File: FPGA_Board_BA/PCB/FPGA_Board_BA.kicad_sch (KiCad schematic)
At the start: 0 parts

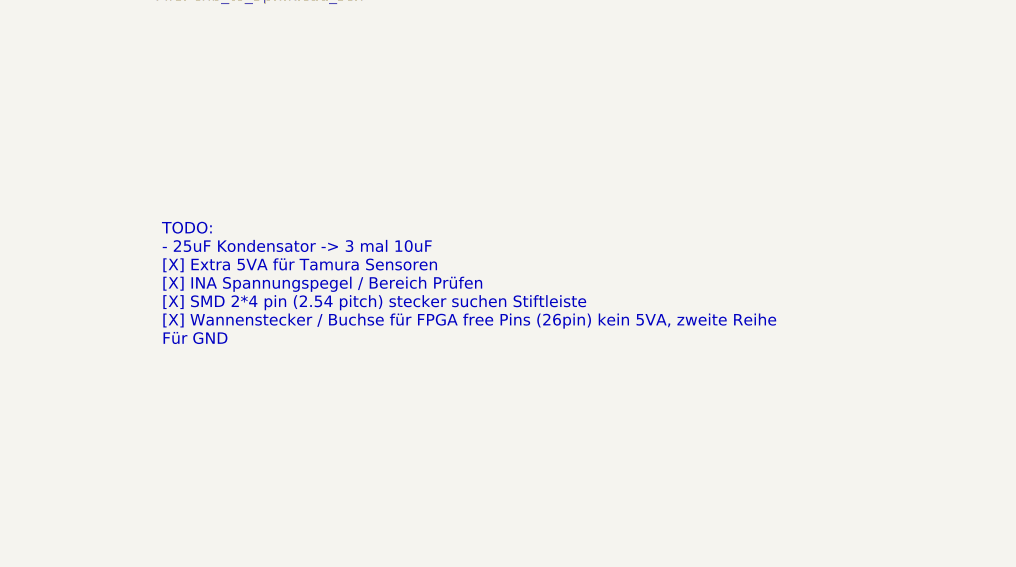
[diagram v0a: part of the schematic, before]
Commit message: started component placement
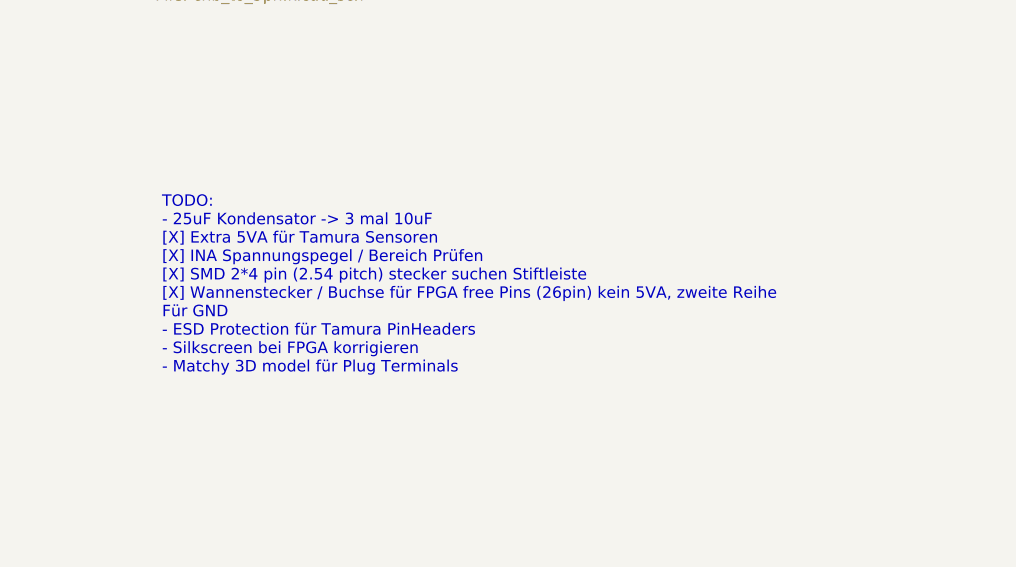
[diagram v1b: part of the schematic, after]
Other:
- note added: "TODO: - 25uF Kondensator -> 3 mal 10uF [X] Extra 5VA für Tamura Sensoren [X] INA Spannungspegel / Bereich Prüfen [X] SMD 2*4 pin (2.54 pitch) stecker suchen Stiftleiste [X] Wannenstecker / Buchse für FPGA free Pins (26pin) kein 5VA, zweite Reihe Für GND - ESD Protection für Tamura PinHeaders - Silkscreen bei FPGA korrigieren - Matchy 3D model für Plug Terminals"
- note removed: "TODO: - 25uF Kondensator -> 3 mal 10uF [X] Extra 5VA für Tamura Sensoren [X] INA Spannungspegel / Bereich Prüfen [X] SMD 2*4 pin (2.54 pitch) stecker suchen Stiftleiste [X] Wannenstecker / Buchse für FPGA free Pins (26pin) kein 5VA, zweite Reihe Für GND"
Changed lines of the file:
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@@
 	(generator_version "9.0")
 	(paper "A3")
-	(text "TODO:\n- 25uF Kondensator -> 3 mal 10uF \n[X] Extra 5VA für Tamura Sensoren\n[X] INA Spannungspegel / Bereich Prüfen\n[X] SMD 2*4 pin (2.54 pitch) stecker suchen Stiftleiste\n[X] Wannenstecker / Buchse für FPGA free Pins (26pin) kein 5VA, zweite Reihe\nFür GND"
+	(text "TODO:\n- 25uF Kondensator -> 3 mal 10uF \n[X] Extra 5VA für Tamura Sensoren\n[X] INA Spannungspegel / Bereich Prüfen\n[X] SMD 2*4 pin (2.54 pitch) stecker suchen Stiftleiste\n[X] Wannenstecker / Buchse für FPGA free Pins (26pin) kein 5VA, zweite Reihe\nFür GND\n- ESD Protection für Tamura PinHeaders\n- Silkscreen bei FPGA korrigieren\n- Matchy 3D model für Plug Terminals"
 		(exclude_from_sim no)
 		(at 328.422 239.268 0)
